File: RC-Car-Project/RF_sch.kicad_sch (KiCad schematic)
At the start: 34 parts

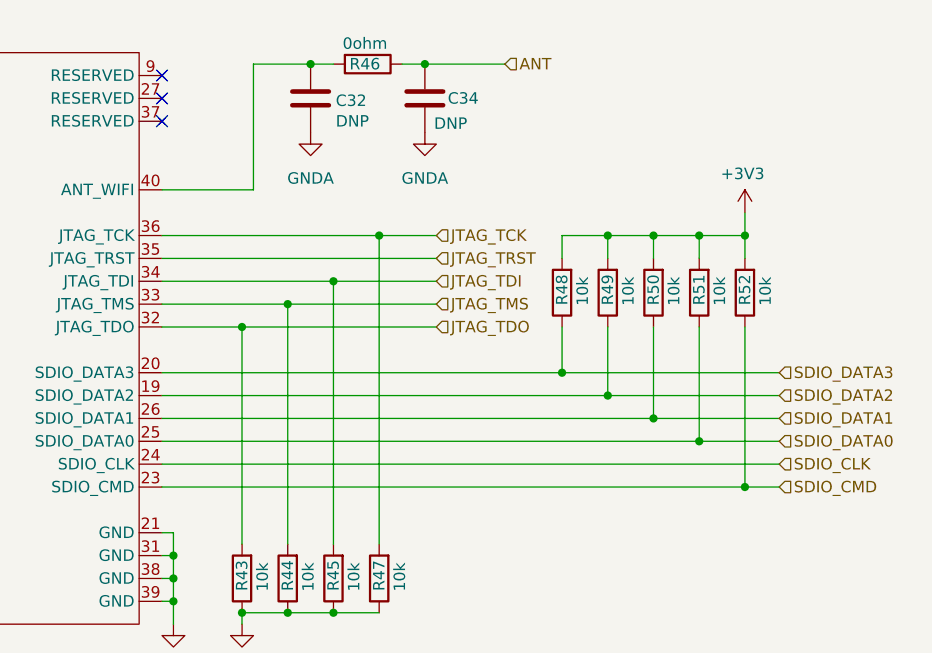
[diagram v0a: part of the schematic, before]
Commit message: Fixed Resistors
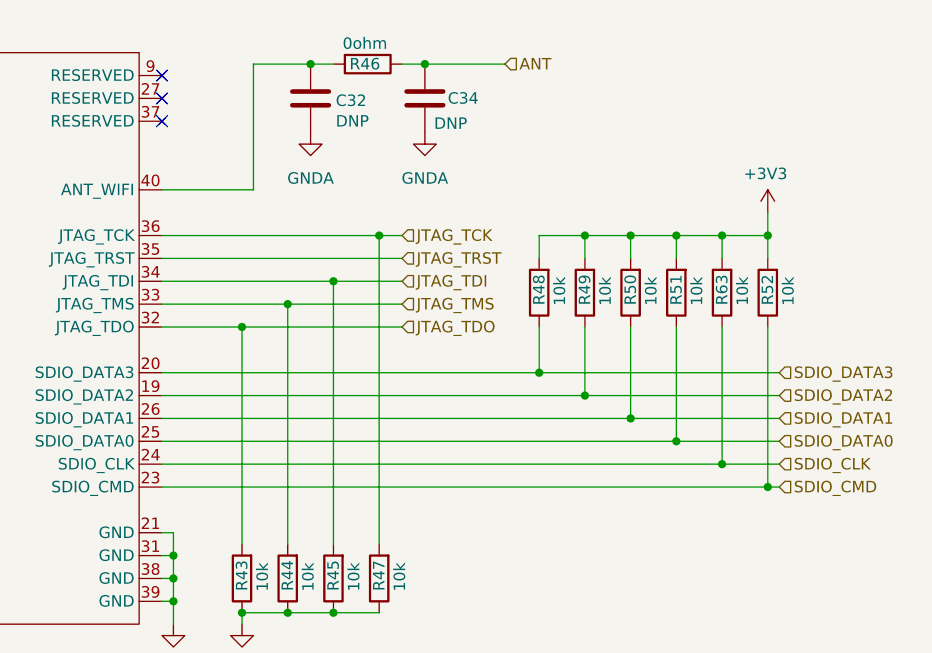
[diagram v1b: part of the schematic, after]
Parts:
- added R63: 10k, Capacitor_SMD:C_0603_1608Metric, symbol Device:R
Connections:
- net +3V3: now also R63.2
- net SDIO_CLK: now also R63.1
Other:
- moved on the sheet: R48, R49, R50, R51, R52
